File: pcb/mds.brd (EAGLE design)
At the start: 50.5 x 49.5 mm, 47 parts, among them IC1 MAX1555, M1 ELECTRET_MICROPHON-F6035AP, U2 ISD1900ISD1932, U5 ATMEGA328

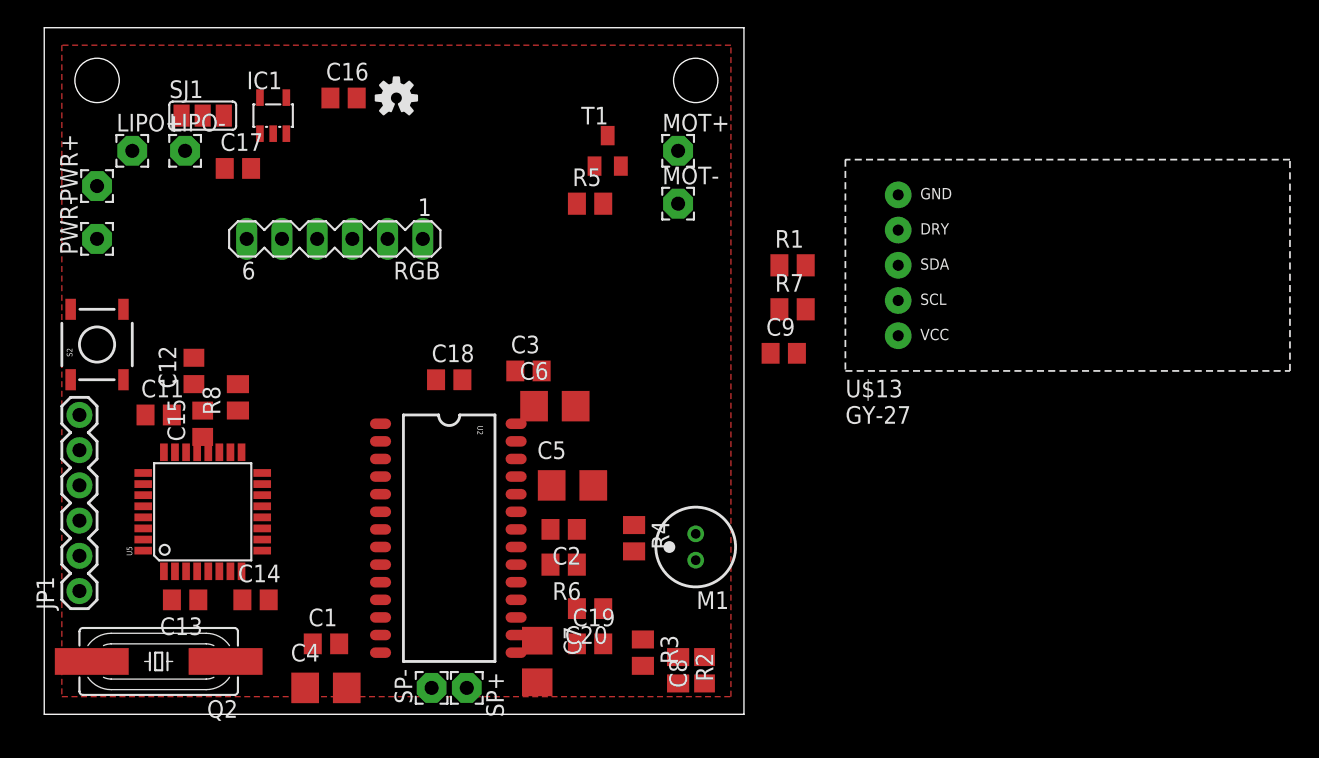
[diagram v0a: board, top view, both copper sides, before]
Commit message: Schema + PCB
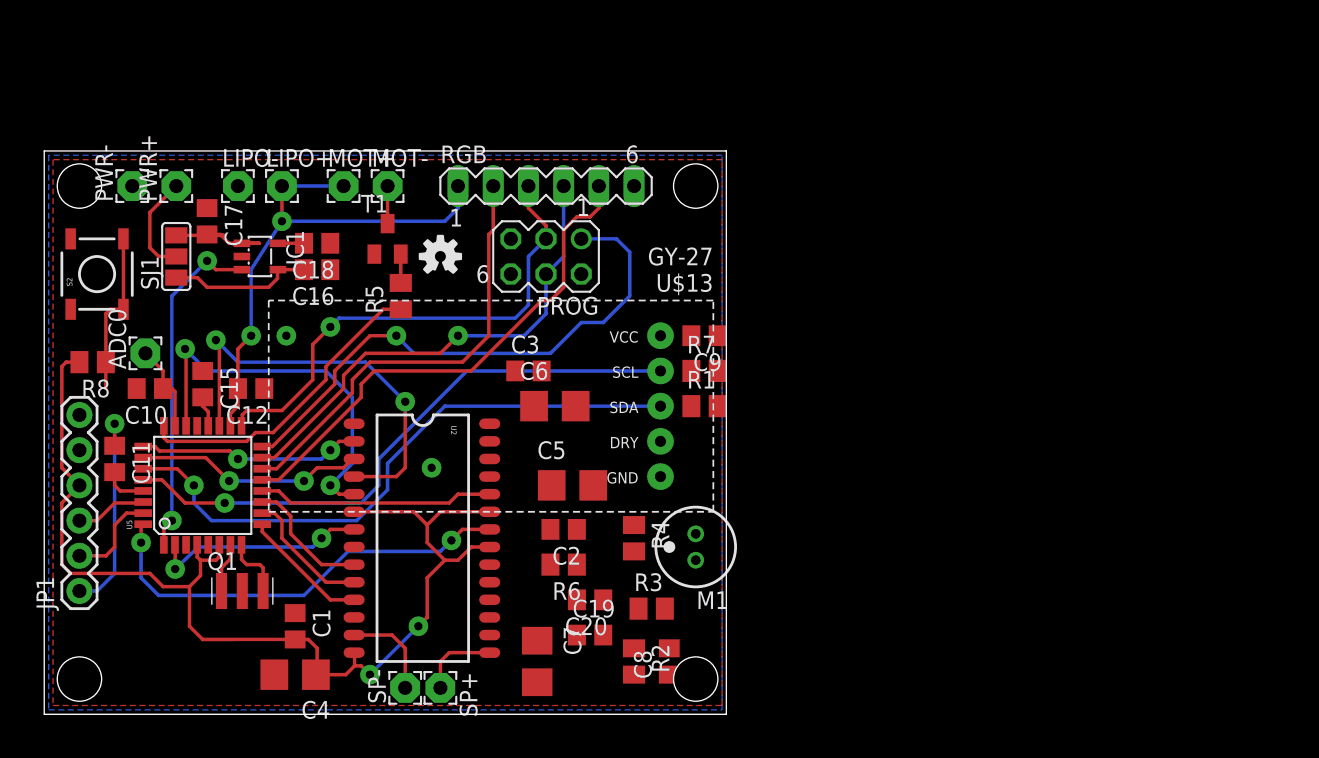
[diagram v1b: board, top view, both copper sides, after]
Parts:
- removed C13, C14: 22pf, rcl:C0805
- removed Q2: (no value), crystal:HC49UP
- added ADC0: (no value), wirepad:2,15/1,0
- added C10: 100nf, rcl:C0805
- added PROG: (no value), con-lstb:MA03-2
- added Q1: CSTCR6M00G53Z, murata-filter:CSTCR6M
- moved MOT+ 24.3 mm to (21.6, 38.1)
- moved MOT- 21.0 mm to (24.8, 38.1)
- moved T1 17.1 mm to (24.8, 34.3)
- moved RGB 15.7 mm to (36.2, 38.1), turned to 0 degrees
- moved R5 15.2 mm to (25.7, 30.2), turned to 90 degrees
- moved C18 13.7 mm to (19.7, 34.0), turned to 180 degrees
- moved C16 12.5 mm to (19.7, 32.1), turned to 180 degrees
- moved R1 12.0 mm to (47.6, 22.2)
- moved U$14 11.9 mm to (28.6, 33.0)
- moved LIPO+ 11.1 mm to (17.1, 38.1)
- moved U$13 10.8 mm to (48.3, 29.8), turned to 180 degrees
- moved R8 10.8 mm to (3.49, 25.4), turned to 180 degrees
- moved SJ1 10.3 mm to (9.53, 33.0), turned to 90 degrees
- moved IC1 10.2 mm to (15.6, 33.0), turned to 270 degrees
- moved R7 7.75 mm to (47.6, 24.8)
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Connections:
- removed net RESET: C11.2, R8.1, S2.3, S2.4, U5.29
- new net ADC0: ADC0.1, C10.1, U5.23
- new net MISO: PROG.1, U5.16
- new net RST: C11.2, PROG.5, R8.1, S2.3, S2.4, U5.29
- net GND: now also C10.2, PROG.6, Q1.2; no longer C13.2, C14.2
- net M6: now also U5.11; no longer U5.9
- net M8: now also U5.9; no longer U5.11
- net MOSI: now also PROG.4
- net N$10: now also Q1.1; no longer C13.1, Q2.2
- net N$9: now also Q1.3; no longer C14.1, Q2.1
- net SCK: now also PROG.3
- net VCC: now also PROG.2
- net VIBRATOR: now also U5.24
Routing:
- net VCC: track 0.00 -> 120.5 mm, vias 0 -> 4
- net SDA: track 0.00 -> 44.1 mm, vias 0 -> 1
- net SCL: track 0.00 -> 43.1 mm, vias 0 -> 1
- net MISO: track 0.00 -> 39.7 mm, vias 0 -> 1
- net SI: track 0.00 -> 37.0 mm
- net SCK: track 0.00 -> 35.8 mm, vias 0 -> 1
- net MOSI: track 0.00 -> 35.1 mm, vias 0 -> 1
- net SS: track 0.00 -> 31.8 mm
- net LED: track 0.00 -> 31.6 mm, vias 0 -> 2
- net M3: track 0.00 -> 30.5 mm, vias 0 -> 2
- net M4: track 0.00 -> 28.1 mm, vias 0 -> 2
- net CHG: track 0.00 -> 24.5 mm, vias 0 -> 2
- net VIBRATOR: track 0.00 -> 22.6 mm
- net REC/PLAY: track 0.00 -> 17.0 mm
- net M2: track 0.00 -> 16.6 mm, vias 0 -> 2
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- added copper zone on layer 16, net GND
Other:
- board size 50.5 x 49.5 mm -> 49.2 x 40.6 mm

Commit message: PCB
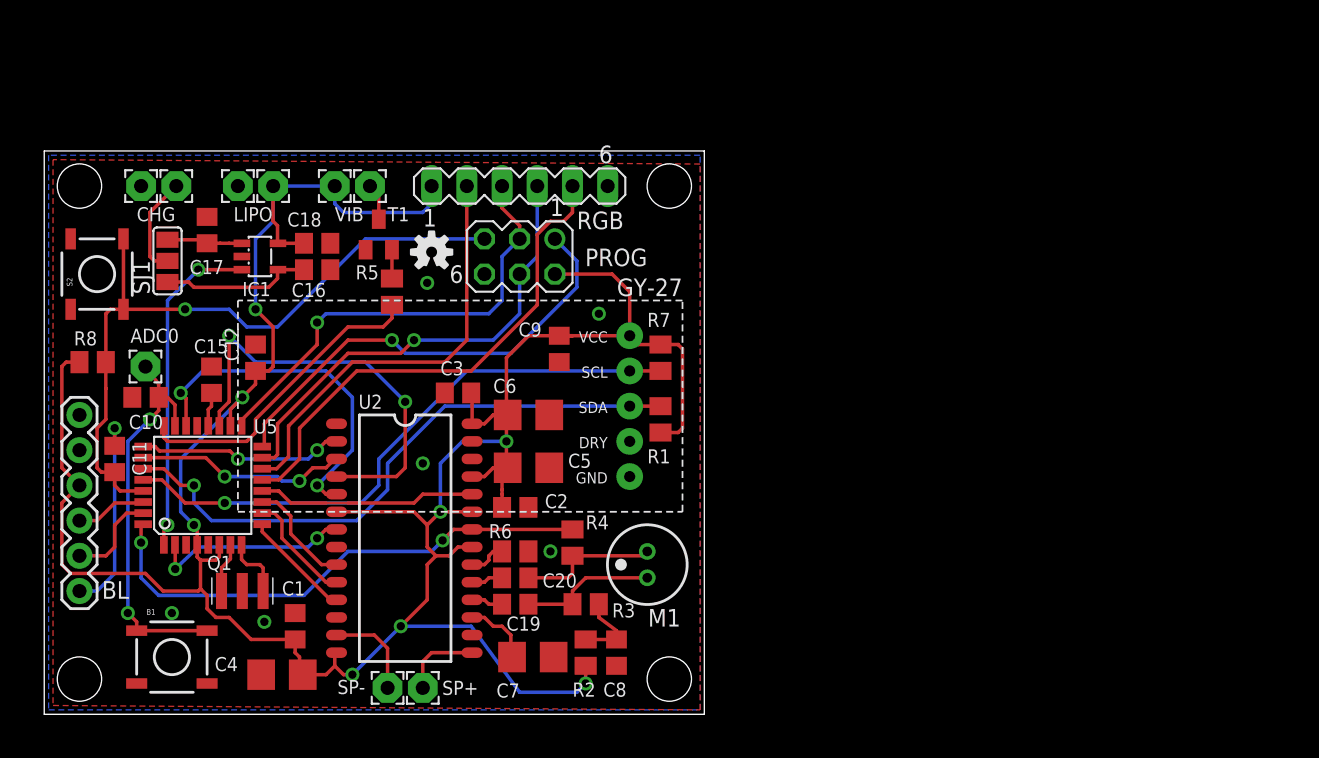
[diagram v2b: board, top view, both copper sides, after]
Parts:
- added B1: Button, SparkFun:TACTILE_SWITCH_SMD
- moved C9 10.5 mm to (37.1, 26.4), turned to 90 degrees
- moved C19 5.84 mm to (34.0, 7.94)
- moved C20 5.63 mm to (34.0, 9.84)
- moved C3 5.32 mm to (29.8, 23.2)
- moved R3 4.77 mm to (39.1, 7.94)
- moved R4 4.46 mm to (38.1, 12.4)
- moved C8 3.86 mm to (41.3, 4.45)
- moved C2 3.84 mm to (34.0, 14.9)
- moved M1 3.72 mm to (43.5, 10.8)
- moved R6 3.62 mm to (34.0, 11.7)
- moved R2 3.55 mm to (39.1, 4.45)
- moved C5 3.42 mm to (34.9, 17.8)
- moved R1 3.31 mm to (44.5, 21.3), turned to 270 degrees
- moved R7 3.31 mm to (44.5, 25.7), turned to 90 degrees
- moved C12 2.25 mm to (15.2, 25.7), turned to 270 degrees
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- renumbered JP1 to BL
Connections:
- net ADC0: now also B1.1, B1.2
- net GND: now also B1.3, B1.4
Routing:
- net VCC: track 120.5 -> 207.9 mm, vias 4 -> 8
- net RST: track 15.1 -> 51.6 mm, vias 0 -> 1
- net ADC0: track 6.49 -> 28.5 mm, vias 0 -> 2
- net N$3: track 0.00 -> 10.1 mm
- net N$2: track 0.00 -> 9.92 mm
- net MISO: track 39.7 -> 33.4 mm
- net LED: track 31.6 -> 37.6 mm
- net AGC: track 0.00 -> 5.64 mm
- net N$6: track 0.00 -> 5.40 mm
- net N$11: track 9.94 -> 5.56 mm
- net SCK: track 35.8 -> 33.0 mm
- net N$1: track 0.00 -> 2.74 mm
- net M4: track 28.1 -> 25.4 mm
- net MIC+: track 0.00 -> 2.29 mm
- net MIC-: track 0.00 -> 2.29 mm
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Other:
- board size 49.2 x 40.6 mm -> 47.6 x 40.6 mm
- board text added: "CHG"
- board text added: "LIPO"
- board text added: "VIB"
